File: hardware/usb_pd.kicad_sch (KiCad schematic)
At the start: 11 parts, among them Q1 STL9P3LLH6, U1 STUSB4500QTR

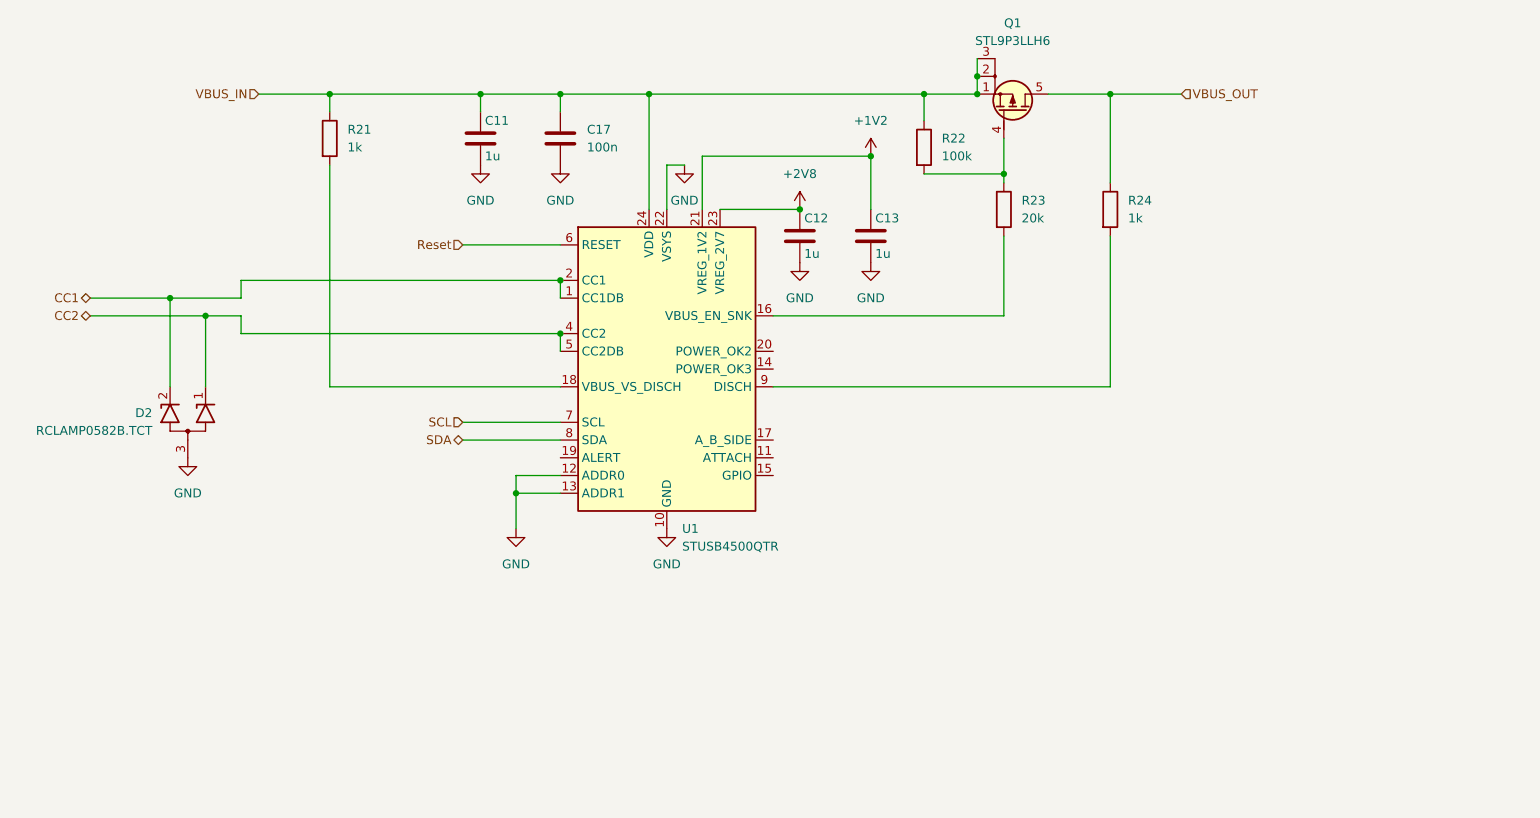
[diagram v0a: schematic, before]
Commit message: Generated first bom
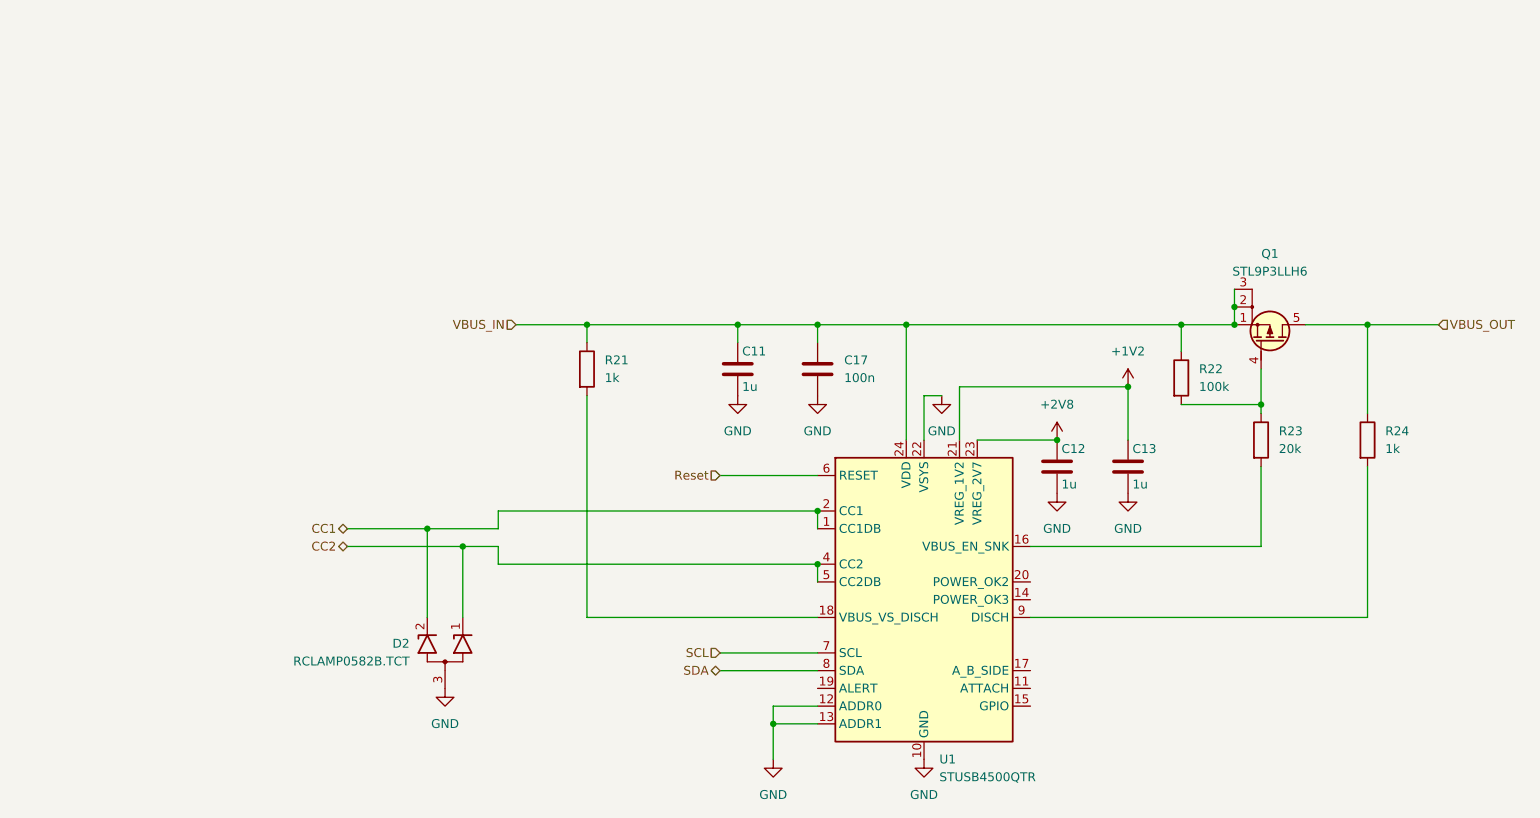
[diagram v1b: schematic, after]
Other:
- moved on the sheet: C11, C12, C13, C17, D2, Q1, R21, R22, R23, R24, U1
